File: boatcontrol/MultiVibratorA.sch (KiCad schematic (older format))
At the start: 5 parts, among them IC401 CD74HCT221E, U2103 74HC86

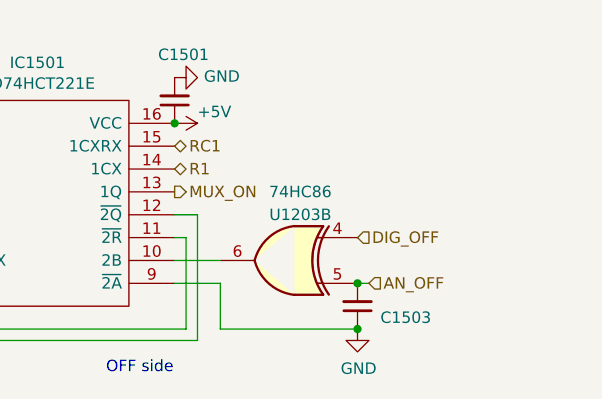
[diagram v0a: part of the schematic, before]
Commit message: Start over
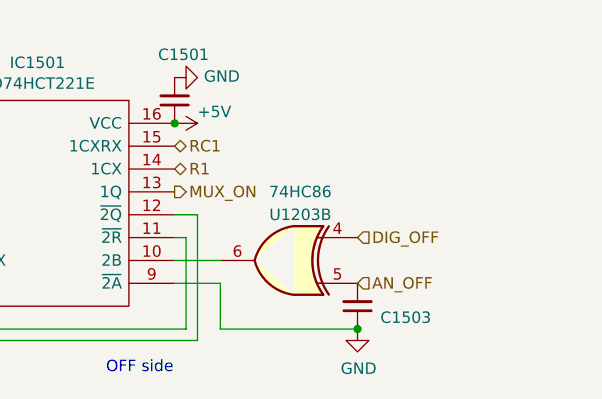
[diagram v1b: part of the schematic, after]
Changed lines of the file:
@@
 Text HLabel 6050 4250 2    50   Output ~ 0
 MUX_ON
-Text HLabel 6900 4650 2    50   Input ~ 0
+Text HLabel 6850 4650 2    50   Input ~ 0
 AN_OFF
 Text HLabel 6850 4450 2    50   Input ~ 0
@@
 	6050 4550 6250 4550
 Wire Wire Line
-	6900 4650 6850 4650
-Connection ~ 6850 4650
-Wire Wire Line
 	6250 4650 6250 4850
